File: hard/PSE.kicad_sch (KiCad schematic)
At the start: 0 parts

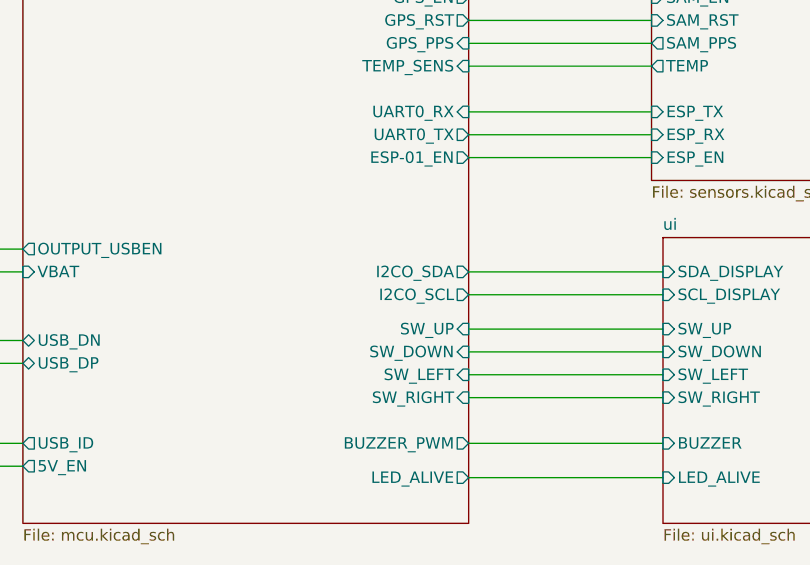
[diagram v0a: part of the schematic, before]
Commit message: update
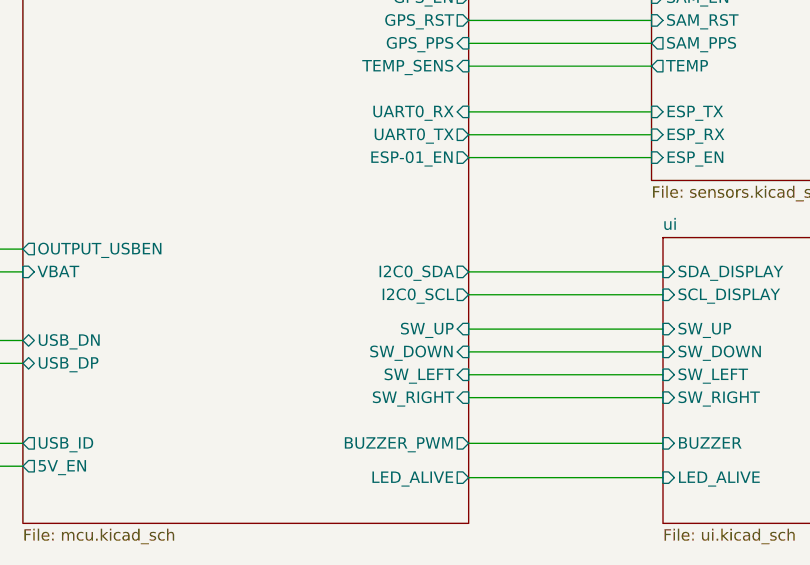
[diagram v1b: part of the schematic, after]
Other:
- sheet mcu ports: added I2C0_SCL, I2C0_SDA; removed I2CO_SCL, I2CO_SDA
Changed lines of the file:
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@@
 			)
 		)
-		(pin "I2CO_SCL" output
+		(pin "I2C0_SCL" output
 			(at 162.56 106.68 0)
 			(effects
@@
 			)
 		)
-		(pin "I2CO_SDA" output
+		(pin "I2C0_SDA" output
 			(at 162.56 104.14 0)
 			(effects
